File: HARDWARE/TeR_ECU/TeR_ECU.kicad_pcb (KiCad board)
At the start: 4 copper layers, 71 parts, among them IC1 MX34040NF2, J1 RJ45_Shielded, J2 RJ45_Shielded, J3 RJ45_Shielded, J4 Debug, Q1 ZXMN3F30FH, Q2 ZXMN3F30FH, SW1 RST, U1 SN65HVD230, U2 SN65HVD230, U3 STM32F446RETx, U4 TSR_1-24120, U5 TSR_1-2450, U6 LM1117MP-3.3, Y1 Crystal

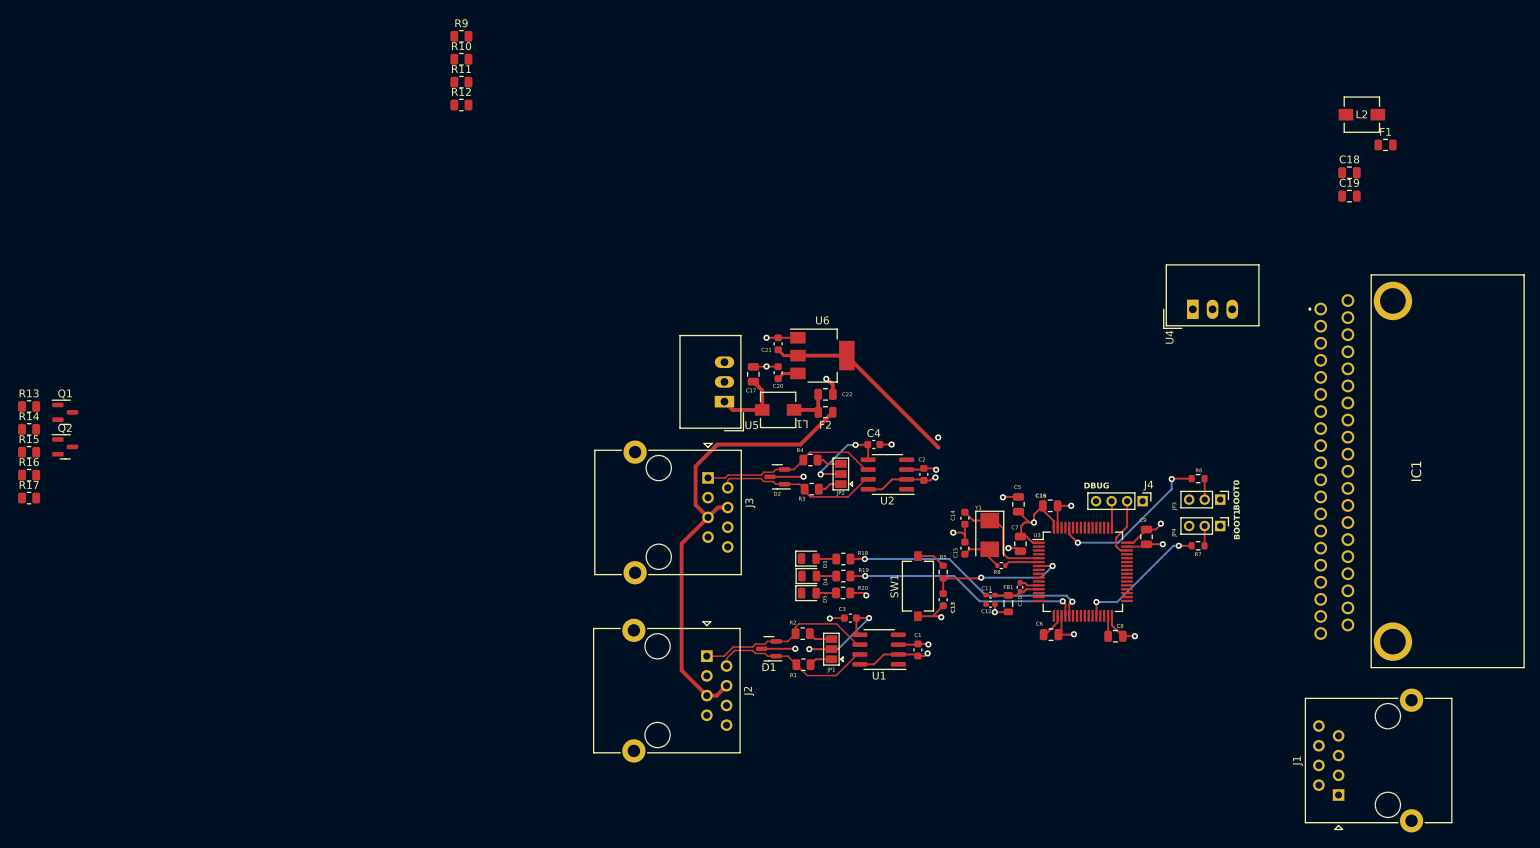
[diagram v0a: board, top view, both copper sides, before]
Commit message: avanzando
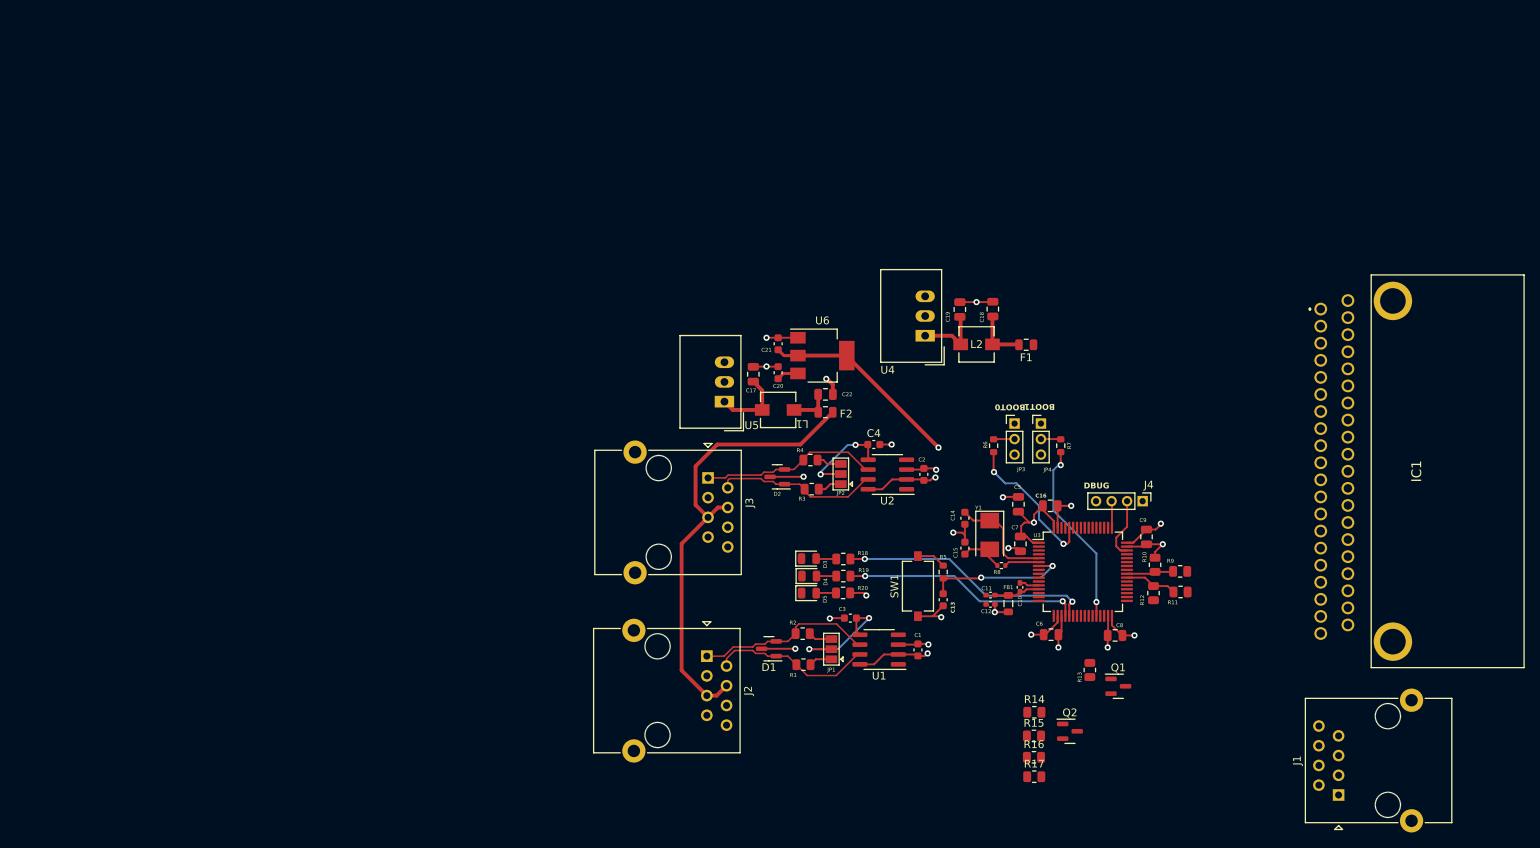
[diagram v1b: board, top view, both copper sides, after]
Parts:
- moved R13 140.8 mm to (152.6, 112.0), turned to 90 degrees
- moved Q1 140.2 mm to (156.3, 114.2)
- moved R14 134.6 mm to (145.4, 117.5)
- moved Q2 134.6 mm to (150.0, 120.0)
- moved R15 134.5 mm to (145.4, 120.5)
- moved R16 134.5 mm to (145.4, 123.3)
- moved R17 134.4 mm to (145.4, 125.8)
- moved R9 115.5 mm to (164.2, 99.3), turned to 180 degrees
- moved R11 113.6 mm to (164.3, 102.0), turned to 180 degrees
- moved R10 110.6 mm to (161.0, 98.5), turned to 90 degrees
- moved R12 109.1 mm to (160.8, 102.2), turned to -90 degrees
- moved L2 57.8 mm to (138.0, 70.1)
- moved F1 53.0 mm to (144.4, 70.2), turned to 180 degrees
- moved C19 52.3 mm to (135.8, 65.6), turned to 90 degrees
- moved C18 49.2 mm to (140.1, 65.5), turned to 90 degrees
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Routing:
- net GND: track 72.4 -> 82.0 mm, vias 15 -> 18
- net Net-(U4-Vin): track 0.00 -> 8.62 mm
- net Net-(C18-Pad1): track 0.00 -> 7.05 mm
- net /Micro/BOOT1: track 17.6 -> 24.5 mm
- net /Detección señales/BSPD_3V3: track 0.00 -> 6.77 mm
- net /Detección señales/TSMS_3V3: track 0.00 -> 6.07 mm
- net /Micro/BOOT0: track 22.0 -> 19.1 mm
